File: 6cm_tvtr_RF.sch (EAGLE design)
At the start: 19 parts

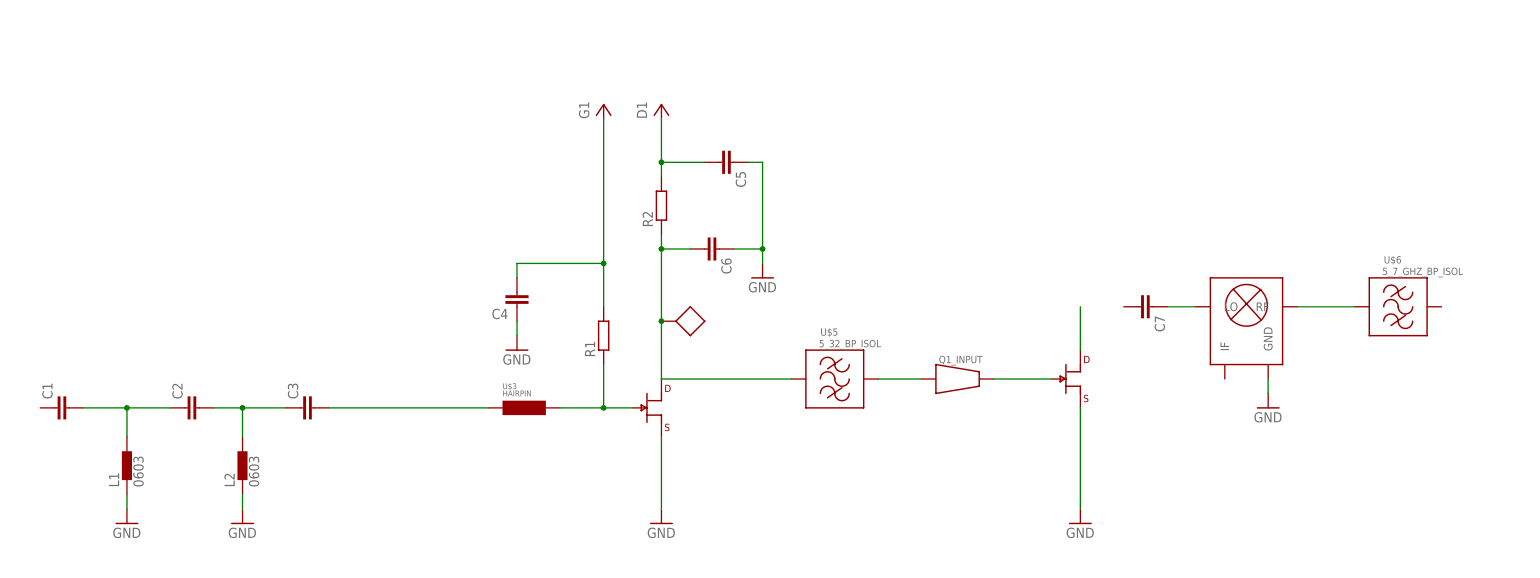
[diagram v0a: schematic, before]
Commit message: layout with GAL1+ etc
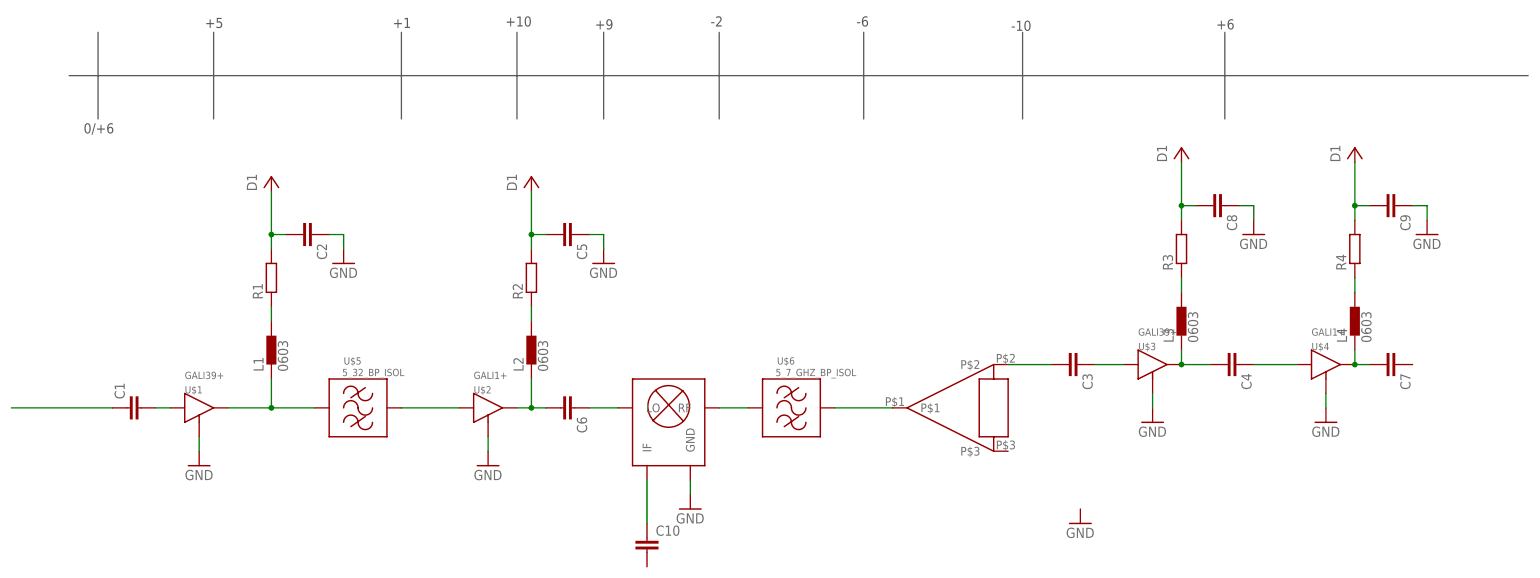
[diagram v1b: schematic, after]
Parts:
- added C10, C8, C9: (no value), rcl:C-EUC0603K
- added L3, L4: 0603, inductors:0603
- added R3, R4: (no value), resistor:R-EU_R0603
- U$1: value CE3512K2 -> GALI39+; device RF:CE3512K2 -> RF:GALI39+
- U$2: value CE3512K2 -> GALI1+; device RF:CE3512K2 -> RF:GALI1+
- U$3: value HAIRPIN -> GALI39+; device RF:HAIRPIN -> RF:GALI39+
- U$4: value 57_FLAKE -> GALI1+; device RF:57_FLAKE -> RF:GALI1+
- U$7: value Q1_INPUT -> 576_WILK; device microstrip:Q1_INPUT -> RF:576_WILK
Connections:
- removed net G1: C4.2, R1.2
- new net N$12: C3.1, U$3.IN
- new net N$13: C4.2, L3.1, U$3.OUT
- new net N$14: C4.1, U$4.IN
- new net N$15: C7.2, L4.1, U$4.OUT
- new net N$16: L3.2, R3.1
- new net N$17: L4.2, R4.1
- new net N$18: C10.1, U$8.IF
- new net N$8: C1.1
- new net VCC: C2.2, R1.2
- net D1: now also C8.2, C9.2, R3.2, R4.2
- net GND: now also C2.1, C8.1, C9.1, U$1.GND, U$2.GND, U$3.GND, U$4.GND; no longer C4.1, C6.1, L1.1, L2.1, U$1.S, U$2.S
- net N$1: now also U$1.IN; no longer C2.1, L1.2
- net N$10: now also C3.2, U$7.P$2; no longer U$2.D
- net N$2: now also R2.1; no longer C2.2, C3.1
- net N$3: now also C6.2, L2.1, U$2.OUT; no longer C3.2, U$3.P$1
- net N$4: now also L1.2; no longer U$1.G, U$3.P$2
- net N$5: now also L1.1, U$1.OUT; no longer C6.2, R2.1, U$1.D, U$4.P$1
- net N$6: now also U$2.IN; no longer U$7.IN
- net N$7: now also U$6.P$2, U$7.P$1; no longer U$2.G, U$7.OUT
- net N$9: now also C6.1; no longer C7.1
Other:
- note added: "+1"
- note added: "+10"
- note added: "+5"
- note added: "+6"
- note added: "+9"
- note added: "-10"
- note added: "-2"
- note added: "-6"
- note added: "0/+6"
- moved on the sheet: C1, C2, C3, C4, C5, C6, C7, L1, L2, R1, R2, U$5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
